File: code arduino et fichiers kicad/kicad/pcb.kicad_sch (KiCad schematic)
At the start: 46 parts, among them J1 Screw_Terminal_01x04, J2 Screw_Terminal_01x03, U1 LMC6482, U2 LMC6482, U3 LMC6482, U4 LMC6482

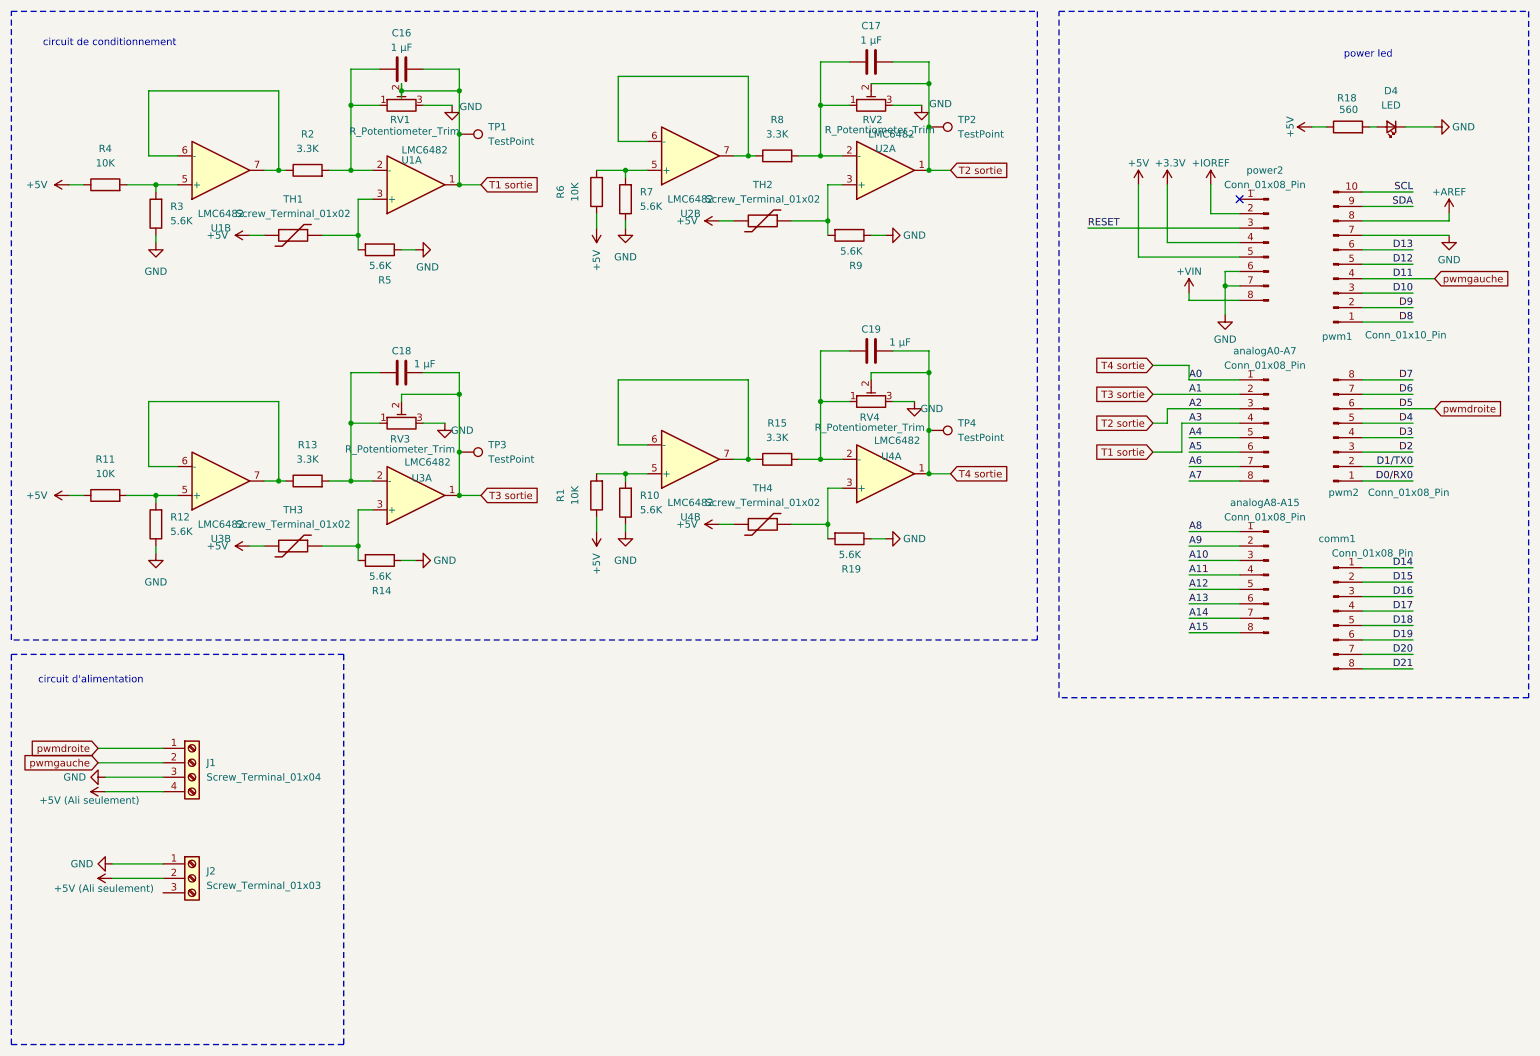
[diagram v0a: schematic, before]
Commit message: PCB V2
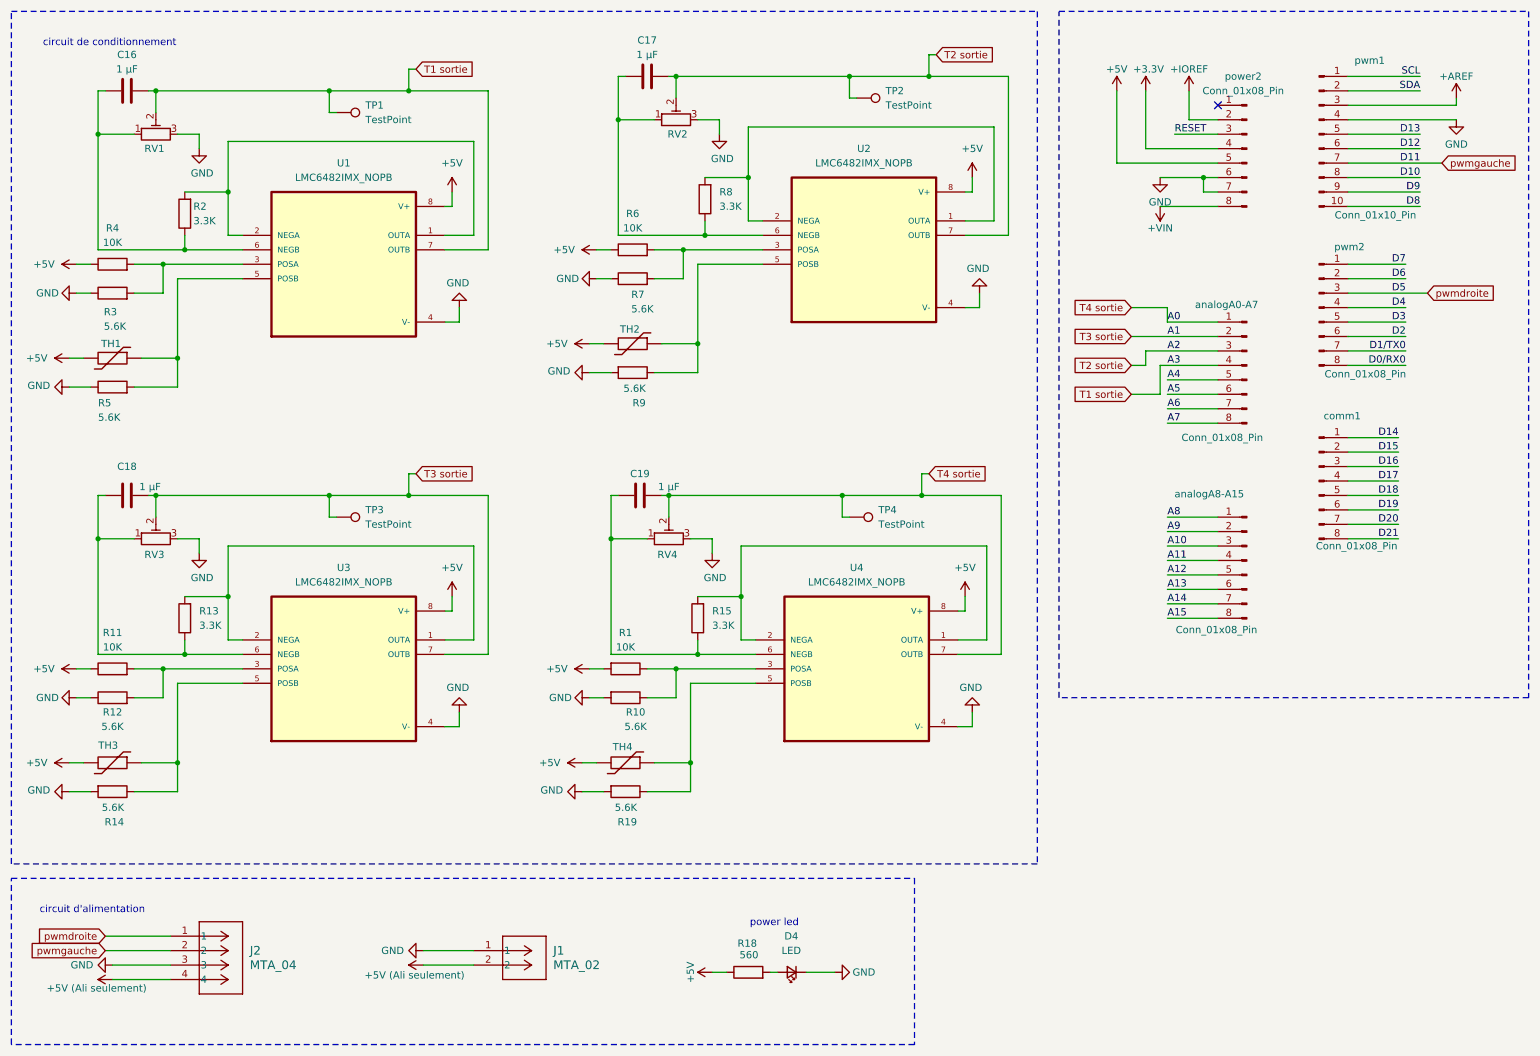
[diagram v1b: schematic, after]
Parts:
- removed J1: Screw_Terminal_01x04, Connector_JST:JST_XH_B4B-XH-A_1x04_P2.50mm_Vertical, symbol Connector:Screw_Terminal_01x04
- removed J2: Screw_Terminal_01x03, Connector_JST:JST_XH_B3B-XH-A_1x03_P2.50mm_Vertical, symbol Connector:Screw_Terminal_01x03
- removed U1, U2, U3, U4: LMC6482, ampli op:LMC6482_SMT, symbol Amplifier_Operational:LMC6482
- added J1: MTA_02, ampli op:MTA_CONN2_640445-2, symbol New_Library:MTA_02
- added J2: MTA_04, ampli op:MTA_CONN4_640445-4, symbol New_Library:MTA_04
- added U1, U2, U3, U4: LMC6482IMX_NOPB, ampli op:LMC6482_SMT, symbol New_Library:LMC6482IMX_NOPB
- TH1, TH2, TH3, TH4: footprint Connector_JST:JST_XH_B2B-XH-A_1x02_P2.50mm_Vertical -> ampli op:MTA_CONN2_640445-2
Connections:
- net +5V: now also R1.2, U1.8 (V+), U2.8 (V+), U3.8 (V+), U4.8 (V+); no longer R1.1
- net +5V (Ali seulement): now also J1.2, J2.4
- net +AREF: now also pwm1.3 (Pin_3); no longer pwm1.8 (Pin_8)
- net D0/RX0: now also pwm2.8 (Pin_8); no longer pwm2.1 (Pin_1)
- net D10: now also pwm1.8 (Pin_8); no longer pwm1.3 (Pin_3)
- net D12: now also pwm1.6 (Pin_6); no longer pwm1.5 (Pin_5)
- net D13: now also pwm1.5 (Pin_5); no longer pwm1.6 (Pin_6)
- net D1/TX0: now also pwm2.7 (Pin_7); no longer pwm2.2 (Pin_2)
- net D2: now also pwm2.6 (Pin_6); no longer pwm2.3 (Pin_3)
- net D3: now also pwm2.5 (Pin_5); no longer pwm2.4 (Pin_4)
- net D4: now also pwm2.4 (Pin_4); no longer pwm2.5 (Pin_5)
- net D6: now also pwm2.2 (Pin_2); no longer pwm2.7 (Pin_7)
- net D7: now also pwm2.1 (Pin_1); no longer pwm2.8 (Pin_8)
- net D8: now also pwm1.10 (Pin_10); no longer pwm1.1 (Pin_1)
- net D9: now also pwm1.9 (Pin_9); no longer pwm1.2 (Pin_2)
- net GND: now also R10.2, R14.2, R19.2, R9.2, pwm1.4 (Pin_4), J1.1, J2.3, U1.4 (V-), U2.4 (V-), U3.4 (V-), U4.4 (V-); no longer R10.1, R14.1, R19.1, R9.1, pwm1.7 (Pin_7)
- net SCL: now also pwm1.1 (Pin_1); no longer pwm1.10 (Pin_10)
- net SDA: now also pwm1.2 (Pin_2); no longer pwm1.9 (Pin_9)
- net T1 sortie: now also U1.7 (OUTB)
- net T2 sortie: now also U2.7 (OUTB)
- net T3 sortie: now also U3.7 (OUTB)
- net T4 sortie: now also U4.7 (OUTB)
- net pwmdroite: now also pwm2.3 (Pin_3), J2.1; no longer pwm2.6 (Pin_6)
- net pwmgauche: now also pwm1.7 (Pin_7), J2.2; no longer pwm1.4 (Pin_4)
- net at C18.1, RV3.1: now also R13.1, U3.6 (NEGB); no longer R13.2
- net at R6.2, R7.2: now also U2.3 (POSA)
- net at R11.2, R12.2: now also U3.3 (POSA)
- net at C19.1, RV4.1: now also R15.1, U4.6 (NEGB); no longer R15.2
- net at C17.1, RV2.1: now also R8.1, U2.6 (NEGB); no longer R8.2
- net at TH2.1: now also R9.1, U2.5 (POSB); no longer R9.2
- net at TH3.1: now also R14.1, U3.5 (POSB); no longer R14.2
- net at TH4.1: now also R19.1, U4.5 (POSB); no longer R19.2
- net at C16.1, RV1.1: now also R2.1, U1.6 (NEGB); no longer R2.2
- net at R5.2, TH1.1: now also U1.5 (POSB)
- net at R3.2, R4.2: now also U1.3 (POSA)
- new net: R15.2, U4.1 (OUTA), U4.2 (NEGA)
- new net: R1.1, R10.1, U4.3 (POSA)
- new net: R13.2, U3.1 (OUTA), U3.2 (NEGA)
- new net: R8.2, U2.1 (OUTA), U2.2 (NEGA)
- new net: R2.2, U1.1 (OUTA), U1.2 (NEGA)
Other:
- moved on the sheet: C16, C17, C18, C19, D4, R1, R10, R11, R12, R13, R14, R15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
